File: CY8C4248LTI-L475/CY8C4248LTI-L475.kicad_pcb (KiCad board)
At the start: 2 copper layers, 28.2 x 28.2 mm, 1 part, among them U1 *

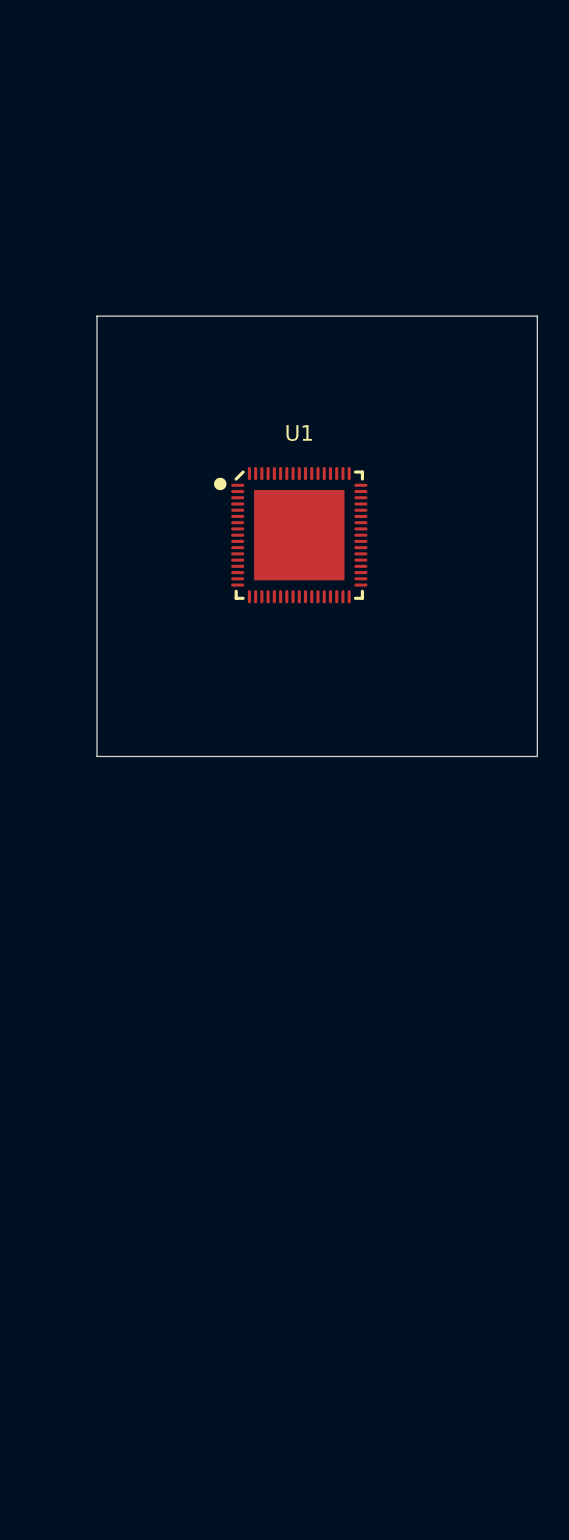
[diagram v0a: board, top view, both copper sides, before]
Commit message: Update
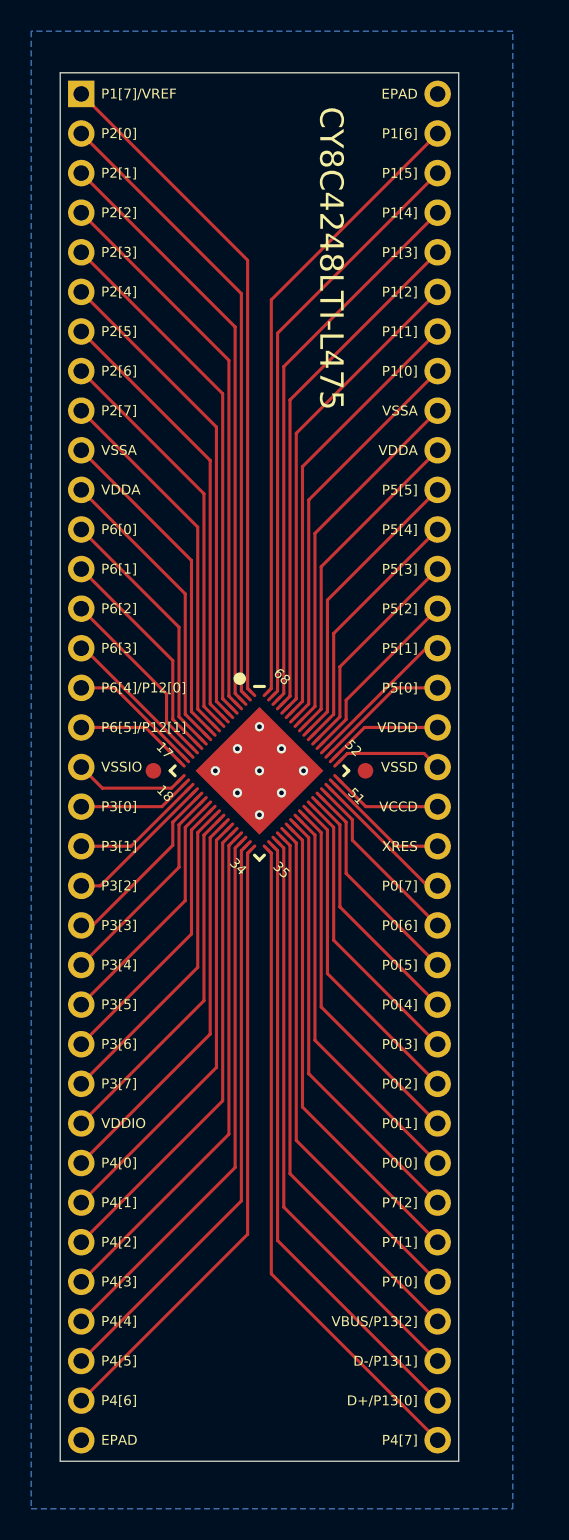
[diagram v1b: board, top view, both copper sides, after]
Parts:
- added J1: Conn_01x35, Connector_PinHeader_2.54mm:PinHeader_1x35_P2.54mm_Vertical, B.Cu at (46.3, 19.6)
- added J2: Conn_01x35, Connector_PinHeader_2.54mm:PinHeader_1x35_P2.54mm_Vertical, B.Cu at (69.1, 105.9)
- moved U1 15.3 mm to (57.7, 63.0), turned to -45 degrees
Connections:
- U1 pad 1: unconnected-(U1-P1_7_VREF-Pad1) -> /P1_7_VREF
- U1 pad 10: unconnected-(U1-VSSA-Pad10) -> /VSSA_0
- U1 pad 11: unconnected-(U1-VDDA-Pad11) -> /VDDA_0
- U1 pad 12: unconnected-(U1-P6_0-Pad12) -> /P6_0
- U1 pad 13: unconnected-(U1-P6_1-Pad13) -> /P6_1
- U1 pad 14: unconnected-(U1-P6_2-Pad14) -> /P6_2
- U1 pad 15: unconnected-(U1-P6_3-Pad15) -> /P6_3
- U1 pad 16: unconnected-(U1-P6_4_P12_0-Pad16) -> /P6_4_P12_0
- U1 pad 17: unconnected-(U1-P6_5_P12_1-Pad17) -> /P6_5_P12_1
- U1 pad 18: unconnected-(U1-VSSIO-Pad18) -> /VSSIO
- U1 pad 19: unconnected-(U1-P3_0-Pad19) -> /P3_0
- U1 pad 2: unconnected-(U1-P2_0-Pad2) -> /P2_0
- U1 pad 20: unconnected-(U1-P3_1-Pad20) -> /P3_1
- U1 pad 21: unconnected-(U1-P3_2-Pad21) -> /P3_2
- U1 pad 22: unconnected-(U1-P3_3-Pad22) -> /P3_3
- U1 pad 23: unconnected-(U1-P3_4-Pad23) -> /P3_4
- U1 pad 24: unconnected-(U1-P3_5-Pad24) -> /P3_5
- U1 pad 25: unconnected-(U1-P3_6-Pad25) -> /P3_6
- U1 pad 26: unconnected-(U1-P3_7-Pad26) -> /P3_7
- U1 pad 27: unconnected-(U1-VDDIO-Pad27) -> /VDDIO
- U1 pad 28: unconnected-(U1-P4_0-Pad28) -> /P4_0
- U1 pad 29: unconnected-(U1-P4_1-Pad29) -> /P4_1
- U1 pad 3: unconnected-(U1-P2_1-Pad3) -> /P2_1
- U1 pad 30: unconnected-(U1-P4_2-Pad30) -> /P4_2
- U1 pad 31: unconnected-(U1-P4_3-Pad31) -> /P4_3
- U1 pad 32: unconnected-(U1-P4_4-Pad32) -> /P4_4
- U1 pad 33: unconnected-(U1-P4_5-Pad33) -> /P4_5
- U1 pad 34: unconnected-(U1-P4_6-Pad34) -> /P4_6
- U1 pad 35: unconnected-(U1-P4_7-Pad35) -> /P4_7
- U1 pad 36: unconnected-(U1-D+_P13_0-Pad36) -> /D+_P13_0
- U1 pad 37: unconnected-(U1-D-_P13_1-Pad37) -> /D-_P13_1
- U1 pad 38: unconnected-(U1-VBUS_P13_2-Pad38) -> /VBUS_P13_2
- U1 pad 39: unconnected-(U1-P7_0-Pad39) -> /P7_0
- U1 pad 4: unconnected-(U1-P2_2-Pad4) -> /P2_2
- U1 pad 40: unconnected-(U1-P7_1-Pad40) -> /P7_1
- U1 pad 41: unconnected-(U1-P7_2-Pad41) -> /P7_2
- U1 pad 42: unconnected-(U1-P0_0-Pad42) -> /P0_0
- U1 pad 43: unconnected-(U1-P0_1-Pad43) -> /P0_1
- U1 pad 44: unconnected-(U1-P0_2-Pad44) -> /P0_2
- U1 pad 45: unconnected-(U1-P0_3-Pad45) -> /P0_3
- U1 pad 46: unconnected-(U1-P0_4-Pad46) -> /P0_4
- U1 pad 47: unconnected-(U1-P0_5-Pad47) -> /P0_5
- U1 pad 48: unconnected-(U1-P0_6-Pad48) -> /P0_6
- U1 pad 49: unconnected-(U1-P0_7-Pad49) -> /P0_7
- U1 pad 5: unconnected-(U1-P2_3-Pad5) -> /P2_3
- U1 pad 50: unconnected-(U1-~{XRES}-Pad50) -> /XRES
- U1 pad 51: unconnected-(U1-VCCD-Pad51) -> /VCCD
- U1 pad 52: unconnected-(U1-VSSD-Pad52) -> /VSSD
- U1 pad 53: unconnected-(U1-VDDD-Pad53) -> /VDDD
- U1 pad 54: unconnected-(U1-P5_0-Pad54) -> /P5_0
- U1 pad 55: unconnected-(U1-P5_1-Pad55) -> /P5_1
- U1 pad 56: unconnected-(U1-P5_2-Pad56) -> /P5_2
- U1 pad 57: unconnected-(U1-P5_3-Pad57) -> /P5_3
- U1 pad 58: unconnected-(U1-P5_4-Pad58) -> /P5_4
- U1 pad 59: unconnected-(U1-P5_5-Pad59) -> /P5_5
- U1 pad 6: unconnected-(U1-P2_4-Pad6) -> /P2_4
- U1 pad 60: unconnected-(U1-VDDA-Pad60) -> /VDDA_1
- U1 pad 61: unconnected-(U1-VSSA-Pad61) -> /VSSA_1
- U1 pad 62: unconnected-(U1-P1_0-Pad62) -> /P1_0
- U1 pad 63: unconnected-(U1-P1_1-Pad63) -> /P1_1
- U1 pad 64: unconnected-(U1-P1_2-Pad64) -> /P1_2
- U1 pad 65: unconnected-(U1-P1_3-Pad65) -> /P1_3
- U1 pad 66: unconnected-(U1-P1_4-Pad66) -> /P1_4
- U1 pad 67: unconnected-(U1-P1_5-Pad67) -> /P1_5
- U1 pad 68: unconnected-(U1-P1_6-Pad68) -> /P1_6
- U1 pad 69: unconnected-(U1-EPAD-Pad69) -> /EPAD
- U1 pad 7: unconnected-(U1-P2_5-Pad7) -> /P2_5
- U1 pad 8: unconnected-(U1-P2_6-Pad8) -> /P2_6
- U1 pad 9: unconnected-(U1-P2_7-Pad9) -> /P2_7
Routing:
- net /P1_7_VREF: track 0.00 -> 42.9 mm
- net /P4_7: track 0.00 -> 42.4 mm
- net /P2_0: track 0.00 -> 40.5 mm
- net /P1_6: track 0.00 -> 40.3 mm
- net /D+_P13_0: track 0.00 -> 40.0 mm
- net /P4_6: track 0.00 -> 39.9 mm
- net /P2_1: track 0.00 -> 38.1 mm
- net /P1_5: track 0.00 -> 38.0 mm
- net /D-_P13_1: track 0.00 -> 37.6 mm
- net /P4_5: track 0.00 -> 37.5 mm
- net /P2_2: track 0.00 -> 35.8 mm
- net /P1_4: track 0.00 -> 35.6 mm
- net /VBUS_P13_2: track 0.00 -> 35.3 mm
- net /P4_4: track 0.00 -> 35.1 mm
- net /P2_3: track 0.00 -> 33.4 mm
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- added copper zone on B.Cu, net /EPAD
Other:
- board size 28.2 x 28.2 mm -> 25.6 x 89.1 mm
- board text added: "CY8C4248LTI-L475"
- board text added: "D+/P13[0]"
- board text added: "D-/P13[1]"
- board text added: "EPAD"
- board text added: "P0[0]"
- board text added: "P0[1]"
- board text added: "P0[2]"
- board text added: "P0[3]"
- board text added: "P0[4]"
- board text added: "P0[5]"
- board text added: "P0[6]"
- board text added: "P0[7]"
- board text added: "P1[0]"
- board text added: "P1[1]"
- board text added: "P1[2]"
- board text added: "P1[3]"
- board text added: "P1[4]"
- board text added: "P1[5]"
- board text added: "P1[6]"
- board text added: "P1[7]/VREF"
- board text added: "P2[0]"
- board text added: "P2[1]"
- board text added: "P2[2]"
- board text added: "P2[3]"
- board text added: "P2[4]"
- board text added: "P2[5]"
- board text added: "P2[6]"
- board text added: "P2[7]"
- board text added: "P3[0]"
- board text added: "P3[1]"
- board text added: "P3[2]"
- board text added: "P3[3]"
- board text added: "P3[4]"
- board text added: "P3[5]"
- board text added: "P3[6]"
- board text added: "P3[7]"
- board text added: "P4[0]"
- board text added: "P4[1]"
- board text added: "P4[2]"
- board text added: "P4[3]"
- board text added: "P4[4]"
- board text added: "P4[5]"
- board text added: "P4[6]"
- board text added: "P4[7]"
- board text added: "P5[0]"
- board text added: "P5[1]"
- board text added: "P5[2]"
- board text added: "P5[3]"
- board text added: "P5[4]"
- board text added: "P5[5]"
- board text added: "P6[0]"
- board text added: "P6[1]"
- board text added: "P6[2]"
- board text added: "P6[3]"
- board text added: "P6[4]/P12[0]"
- board text added: "P6[5]/P12[1]"
- board text added: "P7[0]"
- board text added: "P7[1]"
- board text added: "P7[2]"
- board text added: "VBUS/P13[2]"
- board text added: "VCCD"
- board text added: "VDDA"
- board text added: "VDDD"
- board text added: "VDDIO"
- board text added: "VSSA"
- board text added: "VSSD"
- board text added: "VSSIO"
- board text added: "XRES"
